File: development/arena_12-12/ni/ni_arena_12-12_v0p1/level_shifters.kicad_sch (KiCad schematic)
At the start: 15 parts, among them U1 TXB0108PW, U2 TXB0108PW, U3 TXB0108PW, U4 TXB0108PW, U5 TXB0108PW

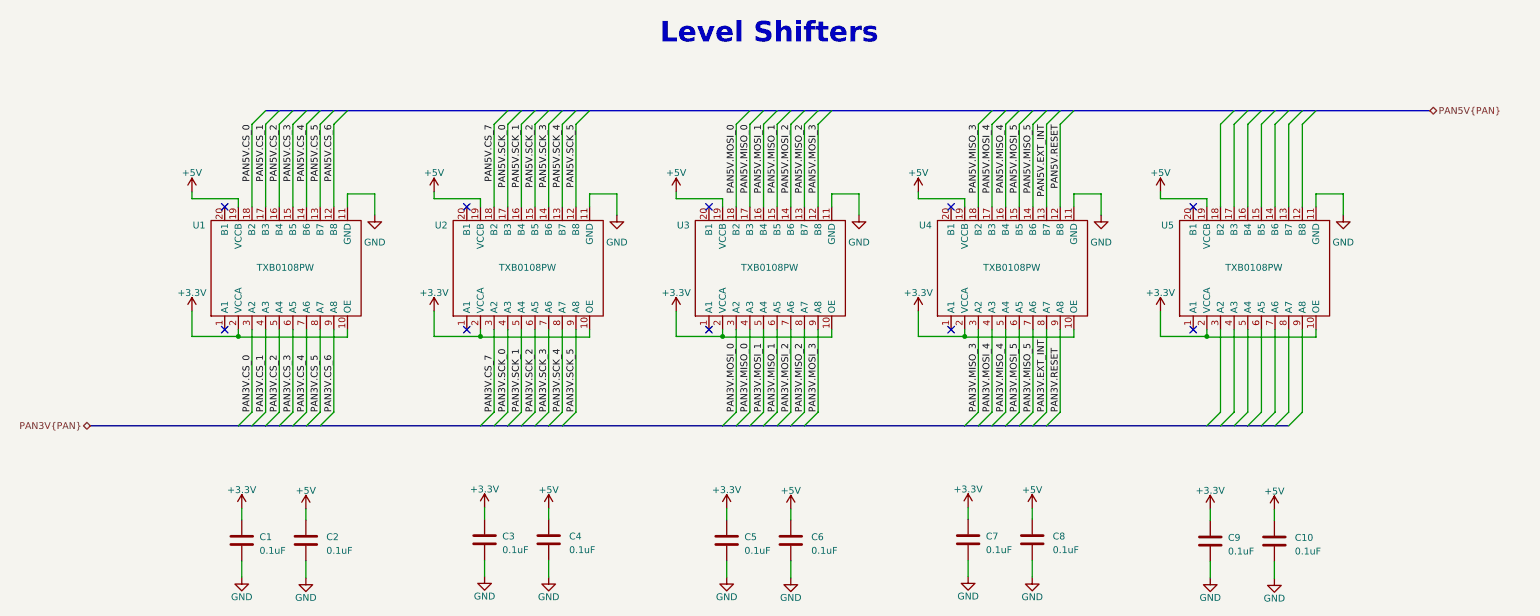
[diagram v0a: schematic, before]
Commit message: Further work on 12-12 ni arena.
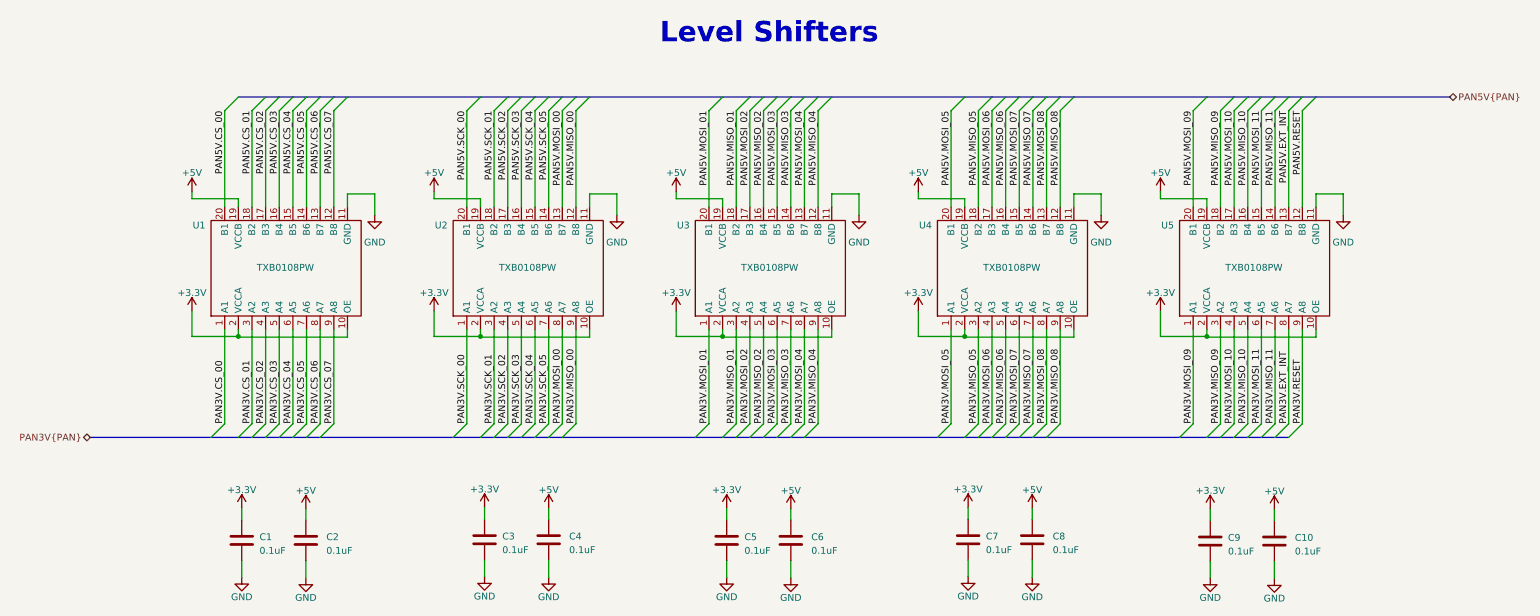
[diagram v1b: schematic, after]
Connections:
- net PAN3V.EXT_INT: now also U5.8 (A7); no longer U4.8 (A7)
- net PAN3V.RESET: now also U5.9 (A8); no longer U4.9 (A8)
- net PAN5V.EXT_INT: now also U5.13 (B7); no longer U4.13 (B7)
- net PAN5V.RESET: now also U5.12 (B8); no longer U4.12 (B8)
- net PAN3V.CS_00: now reaches U1.1 (A1)
- net PAN5V.CS_00: now reaches U1.20 (B1)
- net PAN3V.MOSI_09: now reaches U5.1 (A1)
- net PAN5V.MISO_11: now reaches U5.14 (B6)
- net PAN5V.MOSI_11: now reaches U5.15 (B5)
- net PAN5V.MISO_10: now reaches U5.16 (B4)
- net PAN5V.MOSI_10: now reaches U5.17 (B3)
- net PAN5V.MISO_09: now reaches U5.18 (B2)
- net PAN5V.MOSI_09: now reaches U5.20 (B1)
- net PAN3V.MISO_09: now reaches U5.3 (A2)
- net PAN3V.MOSI_10: now reaches U5.4 (A3)
- net PAN3V.MISO_10: now reaches U5.5 (A4)
- net PAN3V.MOSI_11: now reaches U5.6 (A5)
- net PAN3V.MISO_11: now reaches U5.7 (A6)
- net PAN3V.SCK_00: now reaches U2.1 (A1)
- net PAN5V.SCK_00: now reaches U2.20 (B1)
- net PAN3V.MOSI_01: now reaches U3.1 (A1)
- net PAN5V.MOSI_01: now reaches U3.20 (B1)
- net PAN3V.MOSI_05: now reaches U4.1 (A1)
- net PAN5V.MOSI_05: now reaches U4.20 (B1)
- net PAN3V.CS_0 renamed PAN3V.CS_01
- net PAN3V.CS_1 renamed PAN3V.CS_02
- net PAN3V.CS_2 renamed PAN3V.CS_03
- net PAN3V.CS_3 renamed PAN3V.CS_04
- net PAN3V.CS_4 renamed PAN3V.CS_05
- net PAN3V.CS_5 renamed PAN3V.CS_06
- net PAN3V.CS_6 renamed PAN3V.CS_07
- net PAN3V.CS_7 renamed PAN3V.SCK_01
- net PAN3V.MISO_0 renamed PAN3V.MOSI_02
- net PAN3V.MISO_1 renamed PAN3V.MOSI_03
- net PAN3V.MISO_2 renamed PAN3V.MOSI_04
- net PAN3V.MISO_3 renamed PAN3V.MISO_05
- net PAN3V.MISO_4 renamed PAN3V.MISO_06
- net PAN3V.MISO_5 renamed PAN3V.MISO_07
- net PAN3V.MOSI_0 renamed PAN3V.MISO_01
- net PAN3V.MOSI_1 renamed PAN3V.MISO_02
- net PAN3V.MOSI_2 renamed PAN3V.MISO_03
- net PAN3V.MOSI_3 renamed PAN3V.MISO_04
- net PAN3V.MOSI_4 renamed PAN3V.MOSI_06
- net PAN3V.MOSI_5 renamed PAN3V.MOSI_07
- net PAN3V.SCK_0 renamed PAN3V.SCK_02
- net PAN3V.SCK_1 renamed PAN3V.SCK_03
- net PAN3V.SCK_2 renamed PAN3V.SCK_04
- net PAN3V.SCK_3 renamed PAN3V.SCK_05
- net PAN3V.SCK_4 renamed PAN3V.MOSI_00
- net PAN3V.SCK_5 renamed PAN3V.MISO_00
- net PAN5V.CS_0 renamed PAN5V.CS_01
- net PAN5V.CS_1 renamed PAN5V.CS_02
- net PAN5V.CS_2 renamed PAN5V.CS_03
- net PAN5V.CS_3 renamed PAN5V.CS_04
- net PAN5V.CS_4 renamed PAN5V.CS_05
- net PAN5V.CS_5 renamed PAN5V.CS_06
- net PAN5V.CS_6 renamed PAN5V.CS_07
- net PAN5V.CS_7 renamed PAN5V.SCK_01
- net PAN5V.MISO_0 renamed PAN5V.MOSI_02
- net PAN5V.MISO_1 renamed PAN5V.MOSI_03
- net PAN5V.MISO_2 renamed PAN5V.MOSI_04
- net PAN5V.MISO_3 renamed PAN5V.MISO_05
- net PAN5V.MISO_4 renamed PAN5V.MISO_06
- net PAN5V.MISO_5 renamed PAN5V.MISO_07
- net PAN5V.MOSI_0 renamed PAN5V.MISO_01
- net PAN5V.MOSI_1 renamed PAN5V.MISO_02
- net PAN5V.MOSI_2 renamed PAN5V.MISO_03
- net PAN5V.MOSI_3 renamed PAN5V.MISO_04
- net PAN5V.MOSI_4 renamed PAN5V.MOSI_06
- net PAN5V.MOSI_5 renamed PAN5V.MOSI_07
- net PAN5V.SCK_0 renamed PAN5V.SCK_02
- net PAN5V.SCK_1 renamed PAN5V.SCK_03
- net PAN5V.SCK_2 renamed PAN5V.SCK_04
- net PAN5V.SCK_3 renamed PAN5V.SCK_05
- net PAN5V.SCK_4 renamed PAN5V.MOSI_00
- net PAN5V.SCK_5 renamed PAN5V.MISO_00
- new net PAN3V.MISO_08: U4.9 (A8)
- new net PAN3V.MOSI_08: U4.8 (A7)
- new net PAN5V.MISO_08: U4.12 (B8)
- new net PAN5V.MOSI_08: U4.13 (B7)
- no-connect marks 10 -> 0
